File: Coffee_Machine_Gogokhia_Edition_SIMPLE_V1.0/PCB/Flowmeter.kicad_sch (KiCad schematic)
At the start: 5 parts, among them J7 FLOWMETER

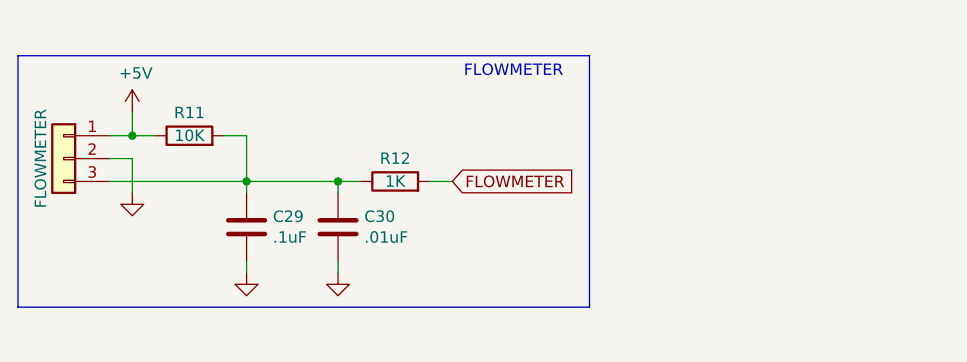
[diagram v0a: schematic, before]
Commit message: 1
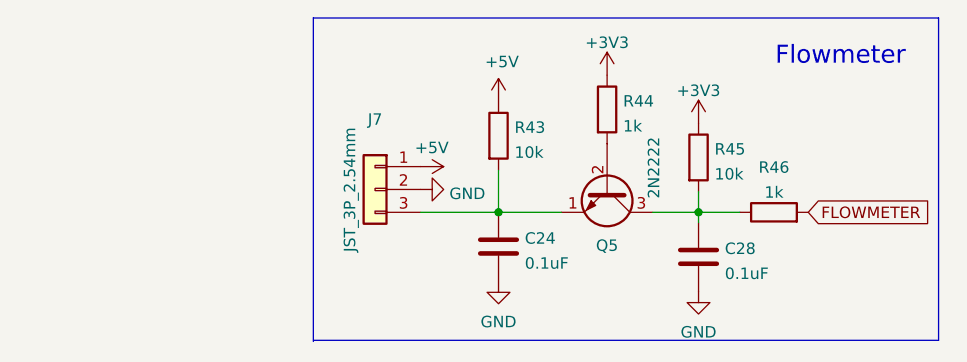
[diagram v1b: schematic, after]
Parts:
- removed C29: .1uF, Capacitor_SMD:C_0603_1608Metric, symbol Device:C
- removed C30: .01uF, Capacitor_SMD:C_0603_1608Metric, symbol Device:C
- removed R11: 10K, Resistor_SMD:R_0603_1608Metric, symbol Device:R
- removed R12: 1K, Resistor_SMD:R_0603_1608Metric, symbol Device:R
- added C24, C28: 0.1uF, Capacitor_SMD:C_0603_1608Metric, symbol Device:C
- added Q5: 2N2222, Package_TO_SOT_SMD:SOT-23, symbol Transistor_BJT:2N2219
- added R43, R45: 10k, Resistor_SMD:R_0603_1608Metric, symbol Device:R
- added R44, R46: 1k, Resistor_SMD:R_0603_1608Metric, symbol Device:R
- J7: value FLOWMETER -> JST_3P_2.54mm
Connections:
- net +5V: now also R43.1
- net FLOWMETER: now also R46.2
- net GND: now also C24.1, C28.1
- net at J7.3 (Pin_3): now also C24.2, Q5.1 (E), R43.2
- new net: Q5.2 (B), R44.2
- new net: C28.2, Q5.3 (C), R45.2, R46.1
- new net +3V3: R44.1, R45.1
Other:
- note added: "Flowmeter"
- note removed: "FLOWMETER"
